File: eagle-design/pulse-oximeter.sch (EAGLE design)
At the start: 9 parts

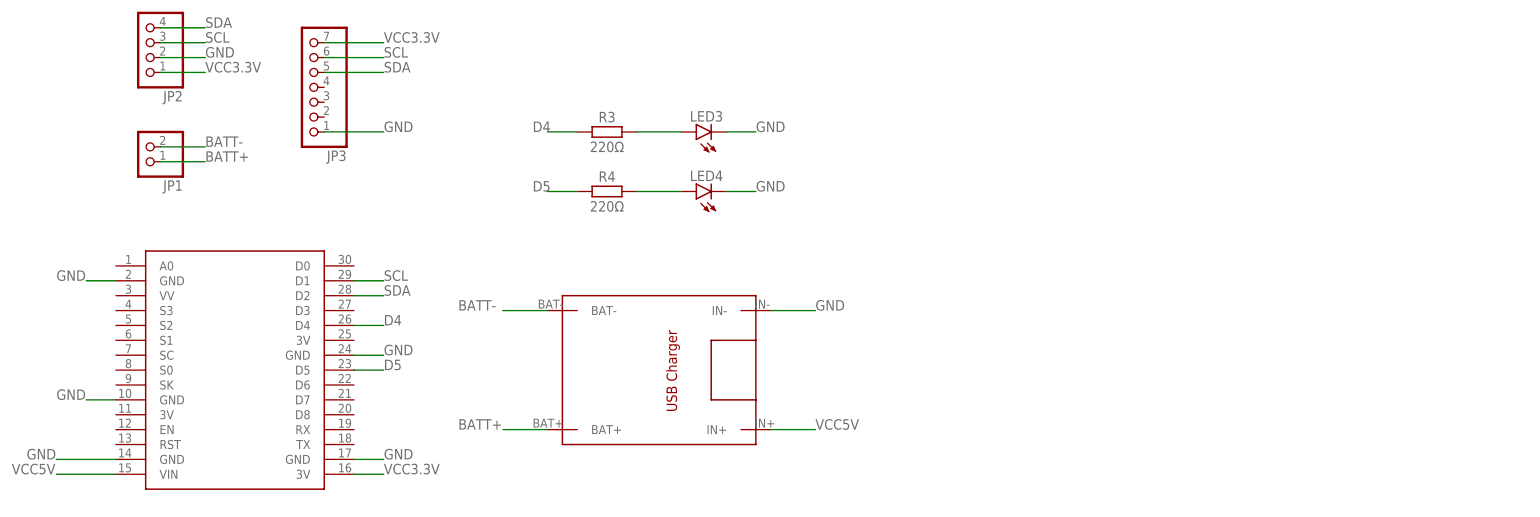
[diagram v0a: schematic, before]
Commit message: Updated design
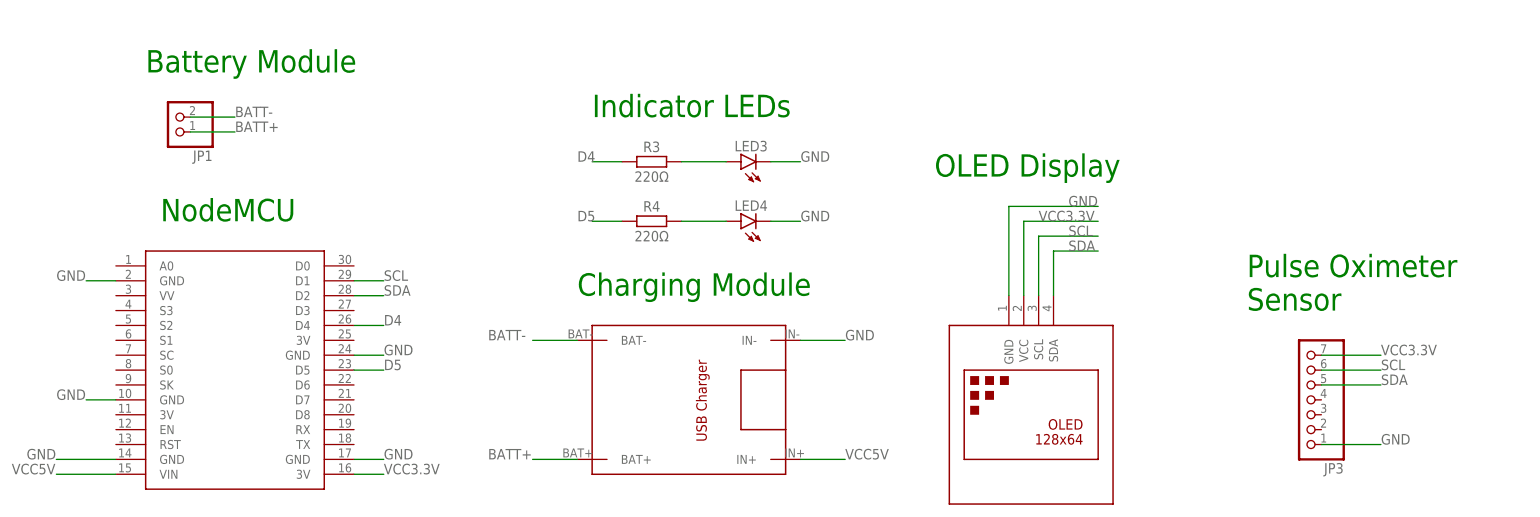
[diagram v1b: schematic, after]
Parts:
- removed JP2: (no value), pinhead:PINHD-1X4
- added U$1: DISPLAY-OLED-128X64-I2C, diy-modules:DISPLAY-OLED-128X64-I2C
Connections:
- net GND: now also U$1.GND; no longer JP2.2
- net SCL: now also U$1.SCL; no longer JP2.3
- net SDA: now also U$1.SDA; no longer JP2.4
- net VCC3.3V: now also U$1.VCC; no longer JP2.1
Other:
- note added: "Battery Module"
- note added: "Charging Module"
- note added: "Indicator LEDs"
- note added: "NodeMCU"
- note added: "OLED Display"
- note added: "Pulse Oximeter Sensor"
- moved on the sheet: JP1, JP3, LED3, LED4, R3, R4
